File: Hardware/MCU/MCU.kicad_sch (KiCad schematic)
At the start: 3 parts, among them J1 Conn_ARM_JTAG_SWD_10, U1 ESP32-S3-WROOM-1

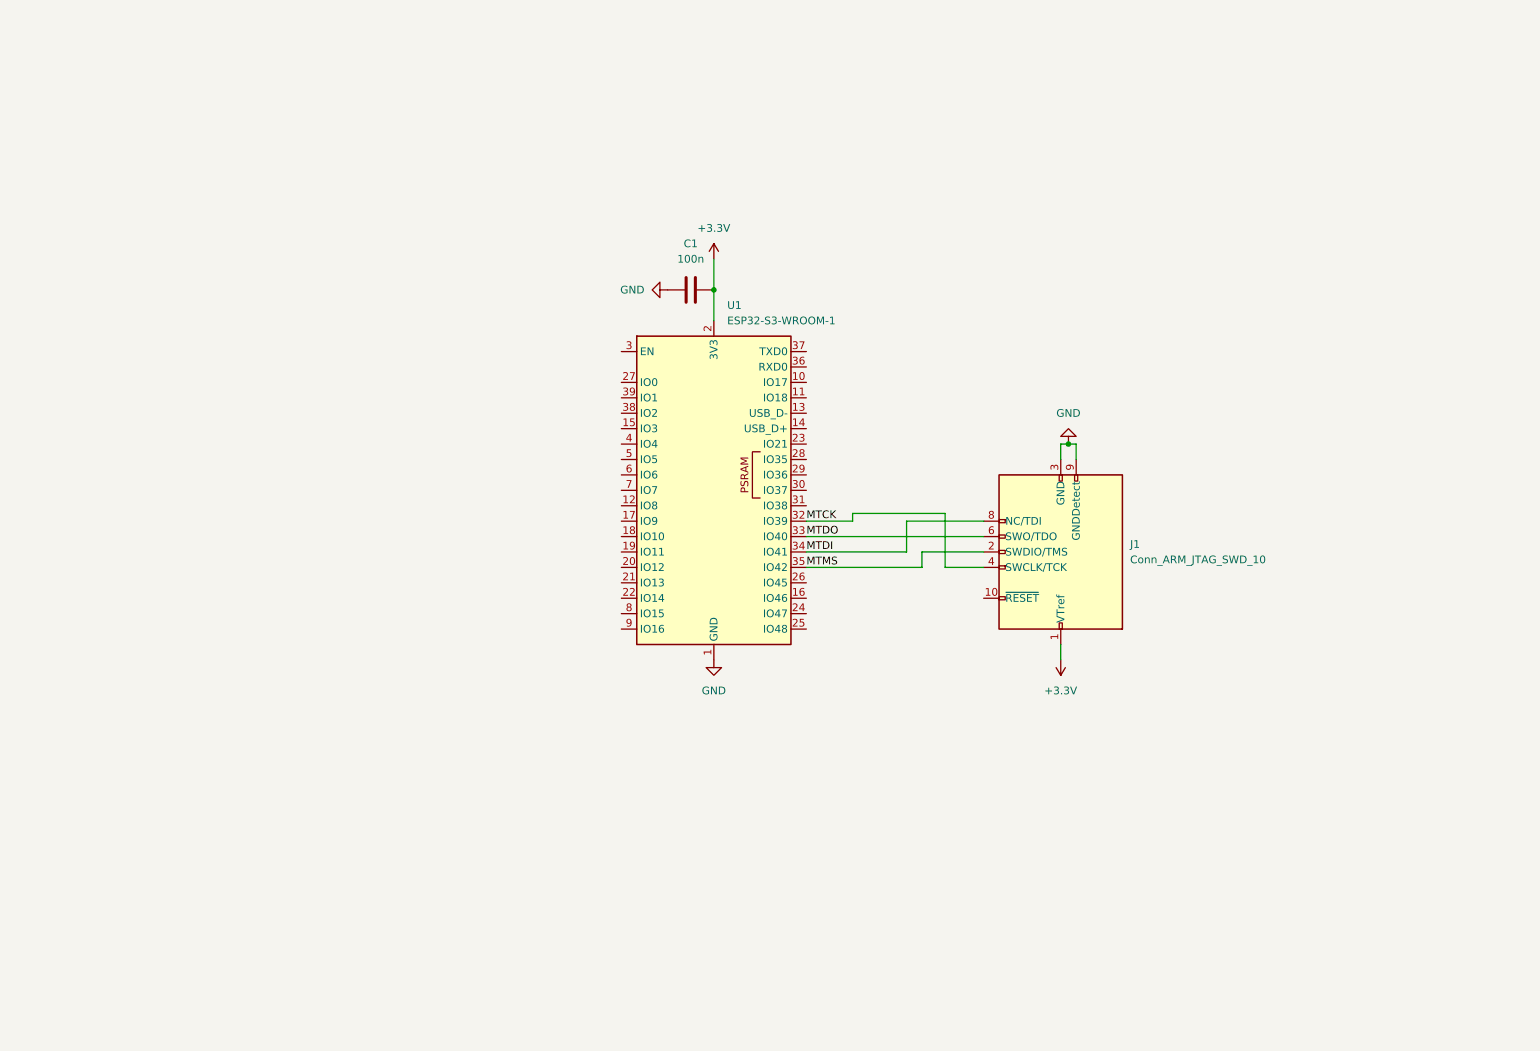
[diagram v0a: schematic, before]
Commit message: MCU schema bijgewerkt
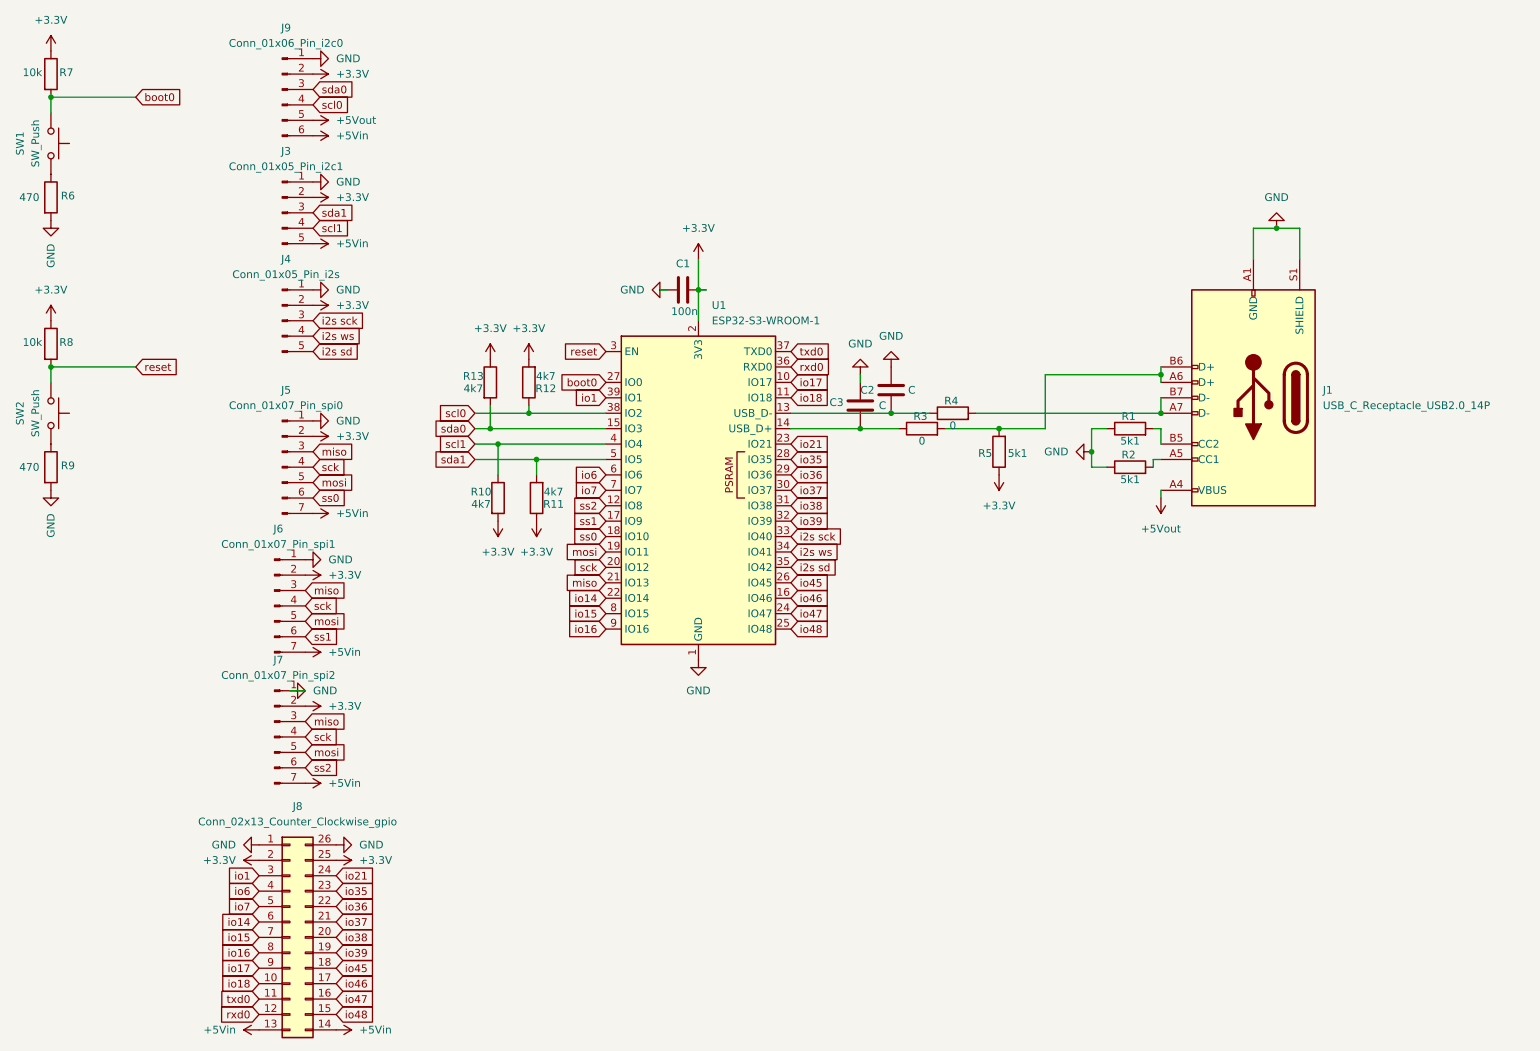
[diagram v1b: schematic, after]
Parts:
- removed J1: Conn_ARM_JTAG_SWD_10, Connector_PinHeader_1.27mm:PinHeader_2x05_P1.27mm_Horizontal, symbol Connector:Conn_ARM_JTAG_SWD_10
- added C2, C3: C, symbol Device:C
- added J1: USB_C_Receptacle_USB2.0_14P, symbol Connector:USB_C_Receptacle_USB2.0_14P
- added J3: Conn_01x05_Pin_i2c1, symbol Connector:Conn_01x05_Pin
- added J4: Conn_01x05_Pin_i2s, symbol Connector:Conn_01x05_Pin
- added J5: Conn_01x07_Pin_spi0, symbol Connector:Conn_01x07_Pin
- added J6: Conn_01x07_Pin_spi1, symbol Connector:Conn_01x07_Pin
- added J7: Conn_01x07_Pin_spi2, symbol Connector:Conn_01x07_Pin
- added J8: Conn_02x13_Counter_Clockwise_gpio, symbol Connector_Generic:Conn_02x13_Counter_Clockwise
- added J9: Conn_01x06_Pin_i2c0, symbol Connector:Conn_01x06_Pin
- added R1, R2, R5: 5k1, symbol Device:R
- added R10, R11, R12, R13: 4k7, symbol Device:R
- added R3, R4: 0, symbol Device:R
- added R6, R9: 470, symbol Device:R
- added R7, R8: 10k, symbol Device:R
- added SW1, SW2: SW_Push, symbol Switch:SW_Push
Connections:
- net +3.3V: now also J3.2 (Pin_2), J4.2 (Pin_2), J5.2 (Pin_2), J6.2 (Pin_2), J7.2 (Pin_2), J8.2 (Pin_2), J8.25 (Pin_25), J9.2 (Pin_2), R10.2, R11.1, R12.2, R13.1, R5.1, R7.1, R8.1
- net GND: now also C2.1, C3.1, J1.A1 (GND), J1.A12 (GND), J1.B1 (GND), J1.B12 (GND), J1.S1 (SHIELD), J3.1 (Pin_1), J4.1 (Pin_1), J5.1 (Pin_1), J6.1 (Pin_1), J7.1 (Pin_1), J8.1 (Pin_1), J8.26 (Pin_26), J9.1 (Pin_1), R1.1, R2.1, R6.2, R9.2
- net io17: now reaches U1.10 (IO17)
- net io17: now also J8.9 (Pin_9)
- net io18: now reaches U1.11 (IO18)
- net io18: now also J8.10 (Pin_10)
- net ss2: now reaches U1.12 (IO8)
- net ss2: now also J7.6 (Pin_6)
- net at U1.13 (USB_D-): now also C2.2, R4.1
- net at U1.14 (USB_D+): now also C3.2, R3.1
- net sda0: now reaches U1.15 (IO3)
- net sda0: now also J9.3 (Pin_3), R13.2
- net io46: now reaches U1.16 (IO46)
- net io46: now also J8.17 (Pin_17)
- net ss1: now reaches U1.17 (IO9)
- net ss1: now also J6.6 (Pin_6)
- net ss0: now reaches U1.18 (IO10)
- net ss0: now also J5.6 (Pin_6)
- net mosi: now reaches U1.19 (IO11)
- net mosi: now also J5.5 (Pin_5), J6.5 (Pin_5), J7.5 (Pin_5)
- net sck: now reaches U1.20 (IO12)
- net sck: now also J5.4 (Pin_4), J6.4 (Pin_4), J7.4 (Pin_4)
- net miso: now reaches U1.21 (IO13)
- net miso: now also J5.3 (Pin_3), J6.3 (Pin_3), J7.3 (Pin_3)
- net io14: now reaches U1.22 (IO14)
- net io14: now also J8.6 (Pin_6)
- net io21: now reaches U1.23 (IO21)
- net io21: now also J8.24 (Pin_24)
- net io47: now reaches U1.24 (IO47)
- net io47: now also J8.16 (Pin_16)
- net io48: now reaches U1.25 (IO48)
- net io48: now also J8.15 (Pin_15)
- net io45: now reaches U1.26 (IO45)
- net io45: now also J8.18 (Pin_18)
- net boot0: now reaches U1.27 (IO0)
- net boot0: now also R7.2, SW1.1
- net io35: now reaches U1.28 (IO35)
- net io35: now also J8.23 (Pin_23)
- net io36: now reaches U1.29 (IO36)
- net io36: now also J8.22 (Pin_22)
- net reset: now reaches U1.3 (EN)
- net reset: now also R8.2, SW2.1
- net io37: now reaches U1.30 (IO37)
- net io37: now also J8.21 (Pin_21)
- net io38: now reaches U1.31 (IO38)
- net io38: now also J8.20 (Pin_20)
- net rxd0: now reaches U1.36 (RXD0)
- net rxd0: now also J8.12 (Pin_12)
- net txd0: now reaches U1.37 (TXD0)
- net txd0: now also J8.11 (Pin_11)
- net scl0: now reaches U1.38 (IO2)
- net scl0: now also J9.4 (Pin_4), R12.1
- net io1: now reaches U1.39 (IO1)
- net io1: now also J8.3 (Pin_3)
- net scl1: now reaches U1.4 (IO4)
- net scl1: now also J3.4 (Pin_4), R10.1
- net sda1: now reaches U1.5 (IO5)
- net sda1: now also J3.3 (Pin_3), R11.2
- net io6: now reaches U1.6 (IO6)
- net io6: now also J8.4 (Pin_4)
- net io7: now reaches U1.7 (IO7)
- net io7: now also J8.5 (Pin_5)
- net io15: now reaches U1.8 (IO15)
- net io15: now also J8.7 (Pin_7)
- net io16: now reaches U1.9 (IO16)
- net io16: now also J8.8 (Pin_8)
- net MTCK renamed io39
- net io39: now also J8.19 (Pin_19)
- net MTDI renamed i2s ws
- net i2s ws: now also J4.4 (Pin_4)
- net MTDO renamed i2s sck
- net i2s sck: now also J4.3 (Pin_3)
- net MTMS renamed i2s sd
- net i2s sd: now also J4.5 (Pin_5)
- new net: J1.A6 (D+), J1.B6 (D+), R3.2, R5.2
- new net: J1.A5 (CC1), R2.2
- new net: J1.A7 (D-), J1.B7 (D-), R4.2
- new net: J1.B5 (CC2), R1.2
- new net: R9.1, SW2.2
- new net: R6.1, SW1.2
- new net +5Vin: J3.5 (Pin_5), J5.7 (Pin_7), J6.7 (Pin_7), J7.7 (Pin_7), J8.13 (Pin_13), J8.14 (Pin_14), J9.6 (Pin_6)
- new net +5Vout: J1.A4 (VBUS), J1.A9 (VBUS), J1.B4 (VBUS), J1.B9 (VBUS), J9.5 (Pin_5)
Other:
- moved on the sheet: C1, U1
